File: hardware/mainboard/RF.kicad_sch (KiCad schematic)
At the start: 39 parts, among them CN4 mmcx, U1 STM32WL33, X2 XTAL_4_PINS

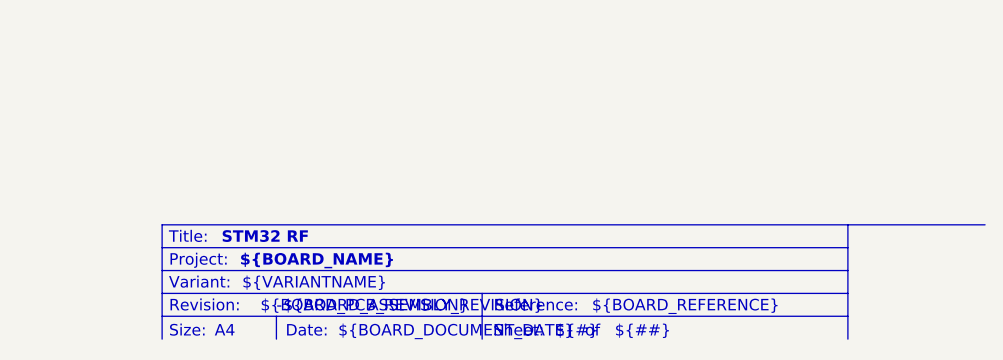
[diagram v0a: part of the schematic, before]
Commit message: latest
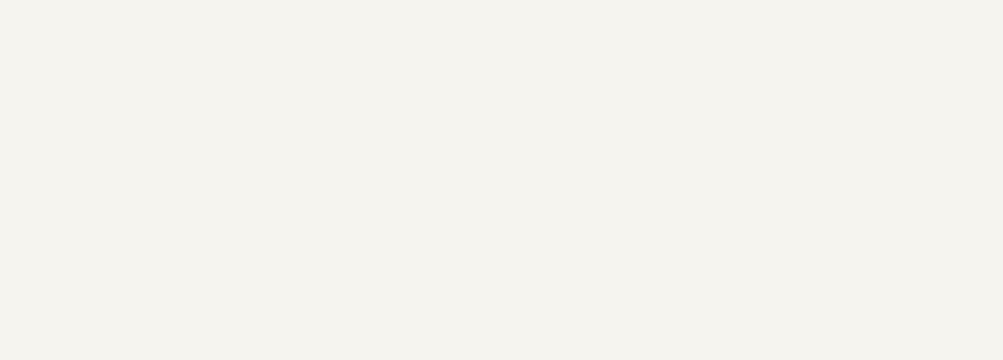
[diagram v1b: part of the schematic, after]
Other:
- note removed: "${##}"
- note removed: "${#}"
- note removed: "${BOARD_ASSEMBLY_REVISION}"
- note removed: "${BOARD_DOCUMENT_DATE}"
- note removed: "${BOARD_NAME}"
- note removed: "${BOARD_PCB_REVISION}"
- note removed: "${BOARD_REFERENCE}"
- note removed: "${TITLE}"
- note removed: "${VARIANTNAME}"
- note removed: "-"
- note removed: "A4"
- note removed: "Date:"
- note removed: "Project:"
- note removed: "Reference:"
- note removed: "Revision:"
- note removed: "Sheet:"
- note removed: "Size:"
- note removed: "Title:"
- note removed: "Variant:"
- note removed: "of"
